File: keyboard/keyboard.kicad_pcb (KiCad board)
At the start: 2 copper layers, 4.5 x 4.5 mm, 141 parts

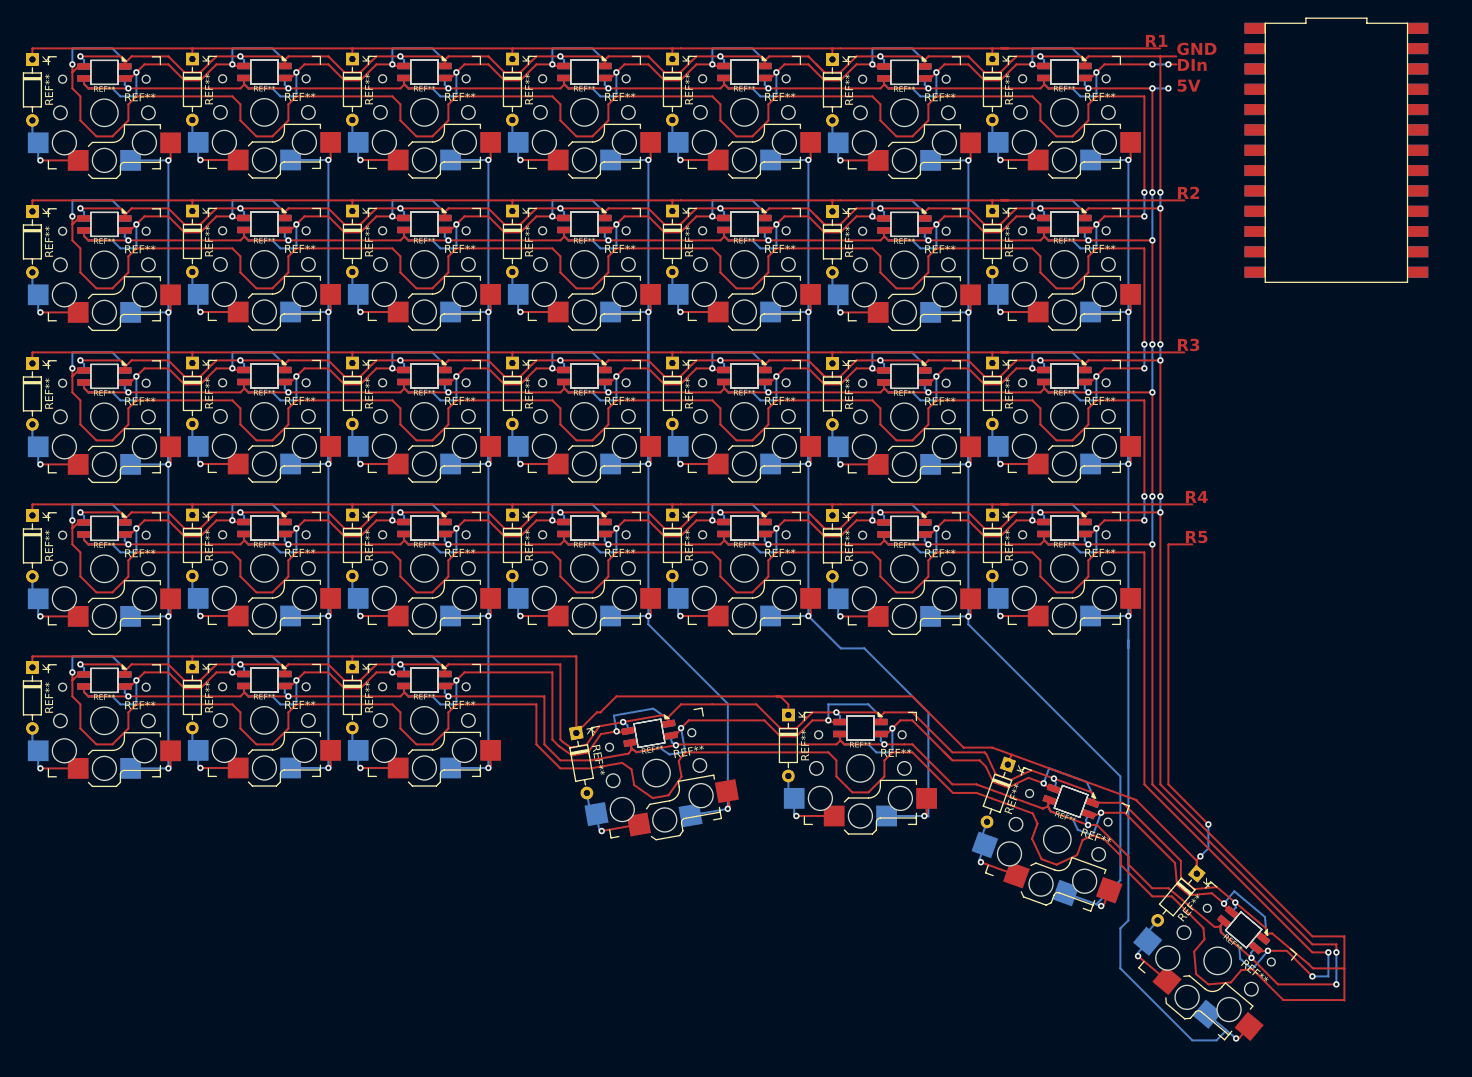
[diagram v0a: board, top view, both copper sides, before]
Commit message: Add files via upload
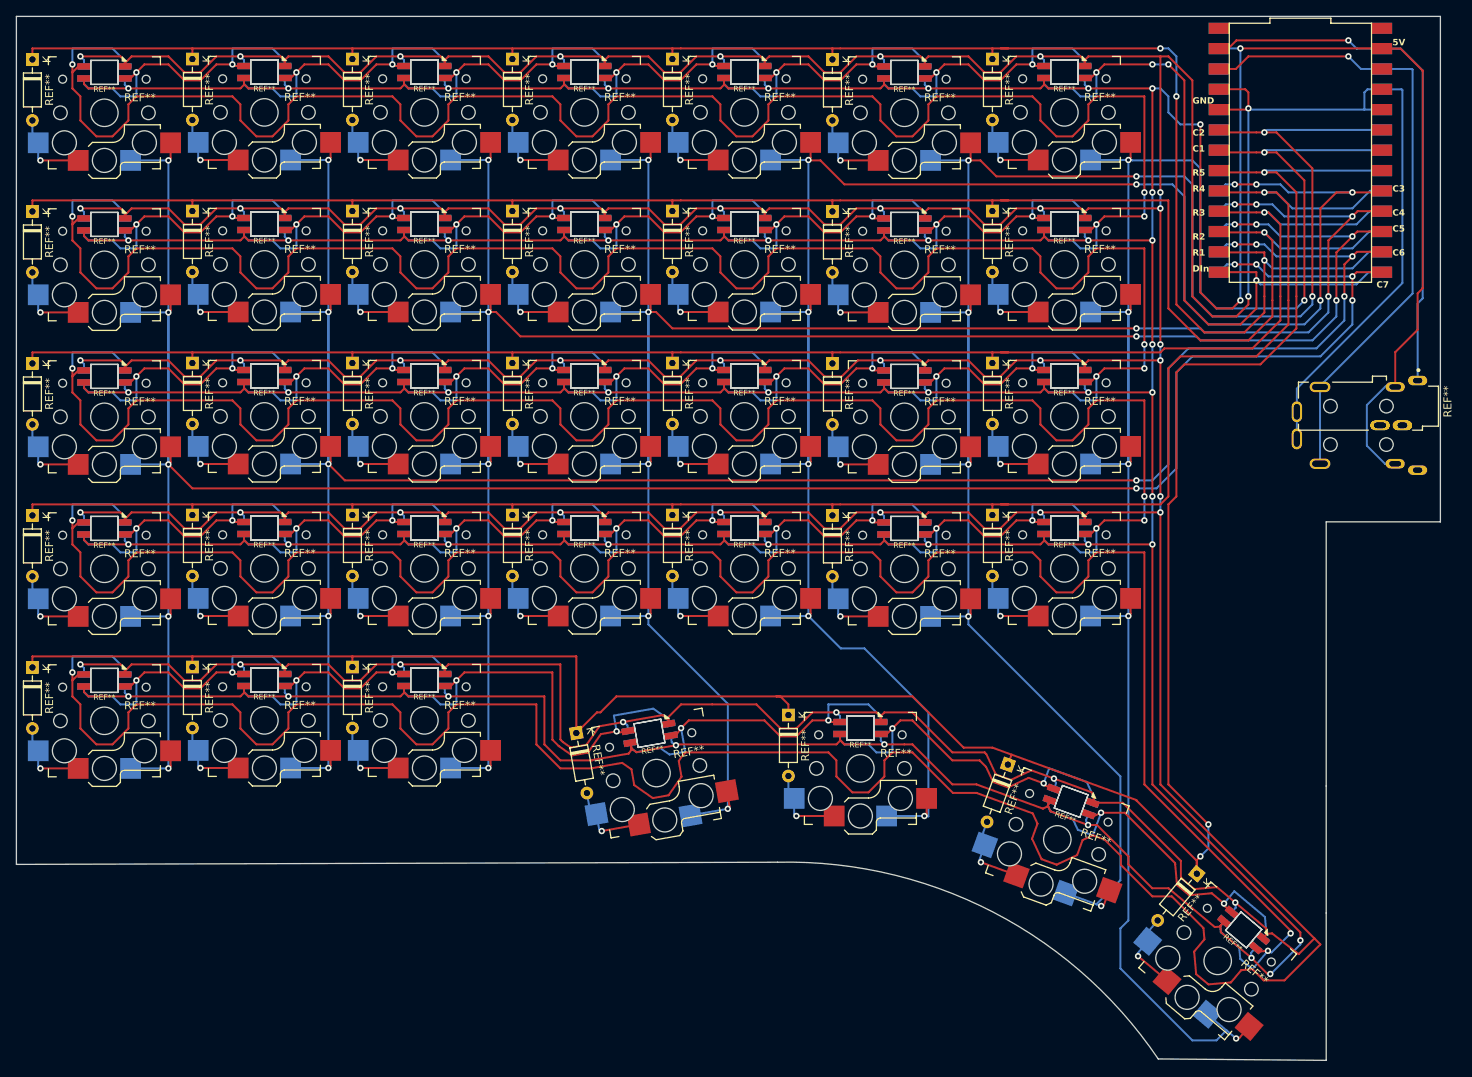
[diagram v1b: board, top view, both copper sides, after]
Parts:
- added REF**: CLIFF_FC68127, FC68127:CLIFF_FC68127, B.Cu at (220.2, 73.5)
- added REF**: CLIFF_FC68127, FC68127:CLIFF_FC68127, F.Cu at (220.3, 68.7)
- moved REF** 4.50 mm to (209.5, 38.0)
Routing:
- net (no net): track 6572.0 -> 8298.2 mm, vias 238 -> 281
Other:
- board size 4.5 x 4.5 mm -> 178 x 130.5 mm
- board text added: "C1"
- board text added: "C2"
- board text added: "C3"
- board text added: "C4"
- board text added: "C5"
- board text added: "C6"
- board text added: "C7"
